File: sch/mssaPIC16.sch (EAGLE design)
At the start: 33 parts, among them IC1 PIC16F676P, IC2 7805L, Q1 BC550C, Q2 BC550C

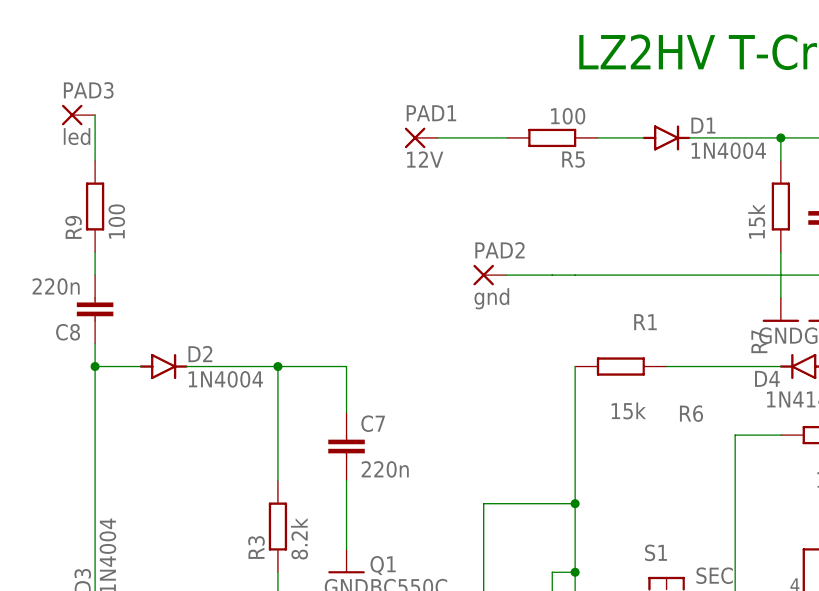
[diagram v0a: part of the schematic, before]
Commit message: Add files via upload
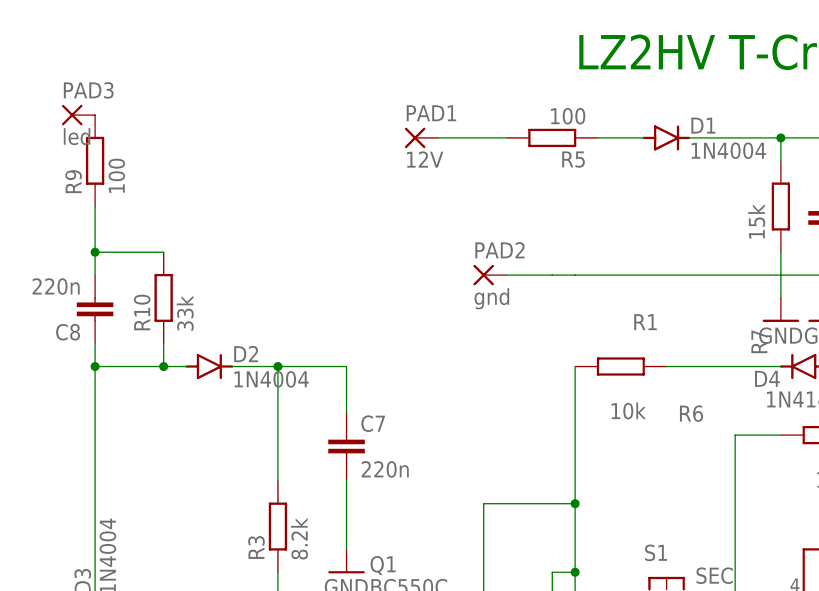
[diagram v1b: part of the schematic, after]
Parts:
- added R10: 33k, rcl:R-EU_0207/2V
- R1: value 15k -> 10k
- R9: device rcl:R-EU_0207/7 -> rcl:R-EU_0207/2V
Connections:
- net N$12: now also R10.2
- net N$13: now also R10.1
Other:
- moved on the sheet: D2, R9
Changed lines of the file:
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@@
 <part name="Q1" library="transistor-npn" library_urn="urn:adsk.eagle:library:398" deviceset="BC550*" device="" package3d_urn="urn:adsk.eagle:package:28989/2" technology="C"/>
 <part name="GND5" library="supply1" deviceset="GND" device=""/>
-<part name="R1" library="rcl" library_urn="urn:adsk.eagle:library:334" deviceset="R-EU_" device="0207/7" package3d_urn="urn:adsk.eagle:package:23493/2" value="15k"/>
+<part name="R1" library="rcl" library_urn="urn:adsk.eagle:library:334" deviceset="R-EU_" device="0207/7" package3d_urn="urn:adsk.eagle:package:23493/2" value="10k"/>
 <part name="R2" library="rcl" library_urn="urn:adsk.eagle:library:334" deviceset="R-EU_" device="0207/7" package3d_urn="urn:adsk.eagle:package:23493/2" value="15k"/>
 <part name="R3" library="rcl" library_urn="urn:adsk.eagle:library:334" deviceset="R-EU_" device="0207/7" package3d_urn="urn:adsk.eagle:package:23493/2" value="8.2k"/>
@@
 <part name="GND17" library="supply1" deviceset="GND" device=""/>
 <part name="D4" library="diode" library_urn="urn:adsk.eagle:library:210" deviceset="1N4148" device="DO35-7" package3d_urn="urn:adsk.eagle:package:43339/2"/>
-<part name="R9" library="rcl" library_urn="urn:adsk.eagle:library:334" deviceset="R-EU_" device="0207/7" package3d_urn="urn:adsk.eagle:package:23493/2" value="100"/>
+<part name="R9" library="rcl" library_urn="urn:adsk.eagle:library:334" deviceset="R-EU_" device="0207/2V" package3d_urn="urn:adsk.eagle:package:23490/1" value="100"/>
+<part name="R10" library="rcl" library_urn="urn:adsk.eagle:library:334" deviceset="R-EU_" device="0207/2V" package3d_urn="urn:adsk.eagle:package:23490/1" value="33k"/>
 </parts>
 <sheets>
@@
 <attribute name="VALUE" x="-2.54" y="50.8" size="1.778" layer="96"/>
 </instance>
-<instance part="D2" gate="1" x="-20.32" y="76.2" smashed="yes">
-<attribute name="NAME" x="-17.78" y="76.6826" size="1.778" layer="95"/>
-<attribute name="VALUE" x="-17.78" y="73.8886" size="1.778" layer="96"/>
+<instance part="D2" gate="1" x="-15.24" y="76.2" smashed="yes">
+<attribute name="NAME" x="-12.7" y="76.6826" size="1.778" layer="95"/>
+<attribute name="VALUE" x="-12.7" y="73.8886" size="1.778" layer="96"/>
 </instance>
 <instance part="D3" gate="1" x="-27.94" y="48.26" smashed="yes" rot="R90">
@@
 <attribute name="VALUE" x="63.5" y="73.4314" size="1.778" layer="96" rot="R180"/>
 </instance>
-<instance part="R9" gate="G$1" x="-27.94" y="93.98" smashed="yes" rot="R90">
-<attribute name="NAME" x="-29.4386" y="90.17" size="1.778" layer="95" rot="R90"/>
-<attribute name="VALUE" x="-24.638" y="90.17" size="1.778" layer="96" rot="R90"/>
+<instance part="R9" gate="G$1" x="-27.94" y="99.06" smashed="yes" rot="R90">
+<attribute name="NAME" x="-29.4386" y="95.25" size="1.778" layer="95" rot="R90"/>
+<attribute name="VALUE" x="-24.638" y="95.25" size="1.778" layer="96" rot="R90"/>
+</instance>
+<instance part="R10" gate="G$1" x="-20.32" y="83.82" smashed="yes" rot="R90">
+<attribute name="NAME" x="-21.8186" y="80.01" size="1.778" layer="95" rot="R90"/>
+<attribute name="VALUE" x="-17.018" y="80.01" size="1.778" layer="96" rot="R90"/>
 </instance>
 </instances>
@@
 <wire x1="0" y1="76.2" x2="-7.62" y2="76.2" width="0.1524" layer="91"/>
 <pinref part="D2" gate="1" pin="C"/>
-<wire x1="-17.78" y1="76.2" x2="-7.62" y2="76.2" width="0.1524" layer="91"/>
+<wire x1="-12.7" y1="76.2" x2="-7.62" y2="76.2" width="0.1524" layer="91"/>
 <junction x="-7.62" y="76.2"/>
 </segment>
@@
 <pinref part="D2" gate="1" pin="A"/>
 <wire x1="-27.94" y1="50.8" x2="-27.94" y2="76.2" width="0.1524" layer="91"/>
-<wire x1="-27.94" y1="76.2" x2="-22.86" y2="76.2" width="0.1524" layer="91"/>
+<wire x1="-27.94" y1="76.2" x2="-20.32" y2="76.2" width="0.1524" layer="91"/>
 <pinref part="C8" gate="G$1" pin="1"/>
+<wire x1="-20.32" y1="76.2" x2="-17.78" y2="76.2" width="0.1524" layer="91"/>
 <wire x1="-27.94" y1="78.74" x2="-27.94" y2="76.2" width="0.1524" layer="91"/>
 <junction x="-27.94" y="76.2"/>
+<pinref part="R10" gate="G$1" pin="1"/>
+<wire x1="-20.32" y1="78.74" x2="-20.32" y2="76.2" width="0.1524" layer="91"/>
+<junction x="-20.32" y="76.2"/>
 </segment>
 </net>
@@
 <pinref part="R9" gate="G$1" pin="1"/>
 <pinref part="C8" gate="G$1" pin="2"/>
+<wire x1="-27.94" y1="93.98" x2="-27.94" y2="88.9" width="0.1524" layer="91"/>
+<pinref part="R10" gate="G$1" pin="2"/>
 <wire x1="-27.94" y1="88.9" x2="-27.94" y2="86.36" width="0.1524" layer="91"/>
+<wire x1="-20.32" y1="88.9" x2="-27.94" y2="88.9" width="0.1524" layer="91"/>
+<junction x="-27.94" y="88.9"/>
 </segment>
 </net>
@@
 <pinref part="R9" gate="G$1" pin="2"/>
 <pinref part="PAD3" gate="P" pin="P"/>
-<wire x1="-27.94" y1="99.06" x2="-27.94" y2="104.14" width="0.1524" layer="91"/>
-</segment>
-</net>
+</segment>
+</net>
